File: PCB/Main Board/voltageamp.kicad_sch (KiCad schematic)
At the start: 45 parts, among them U601 INA828D, U602 DG201, U603 OPA2197xD, U604 DG201, U605 OPA2376xxD

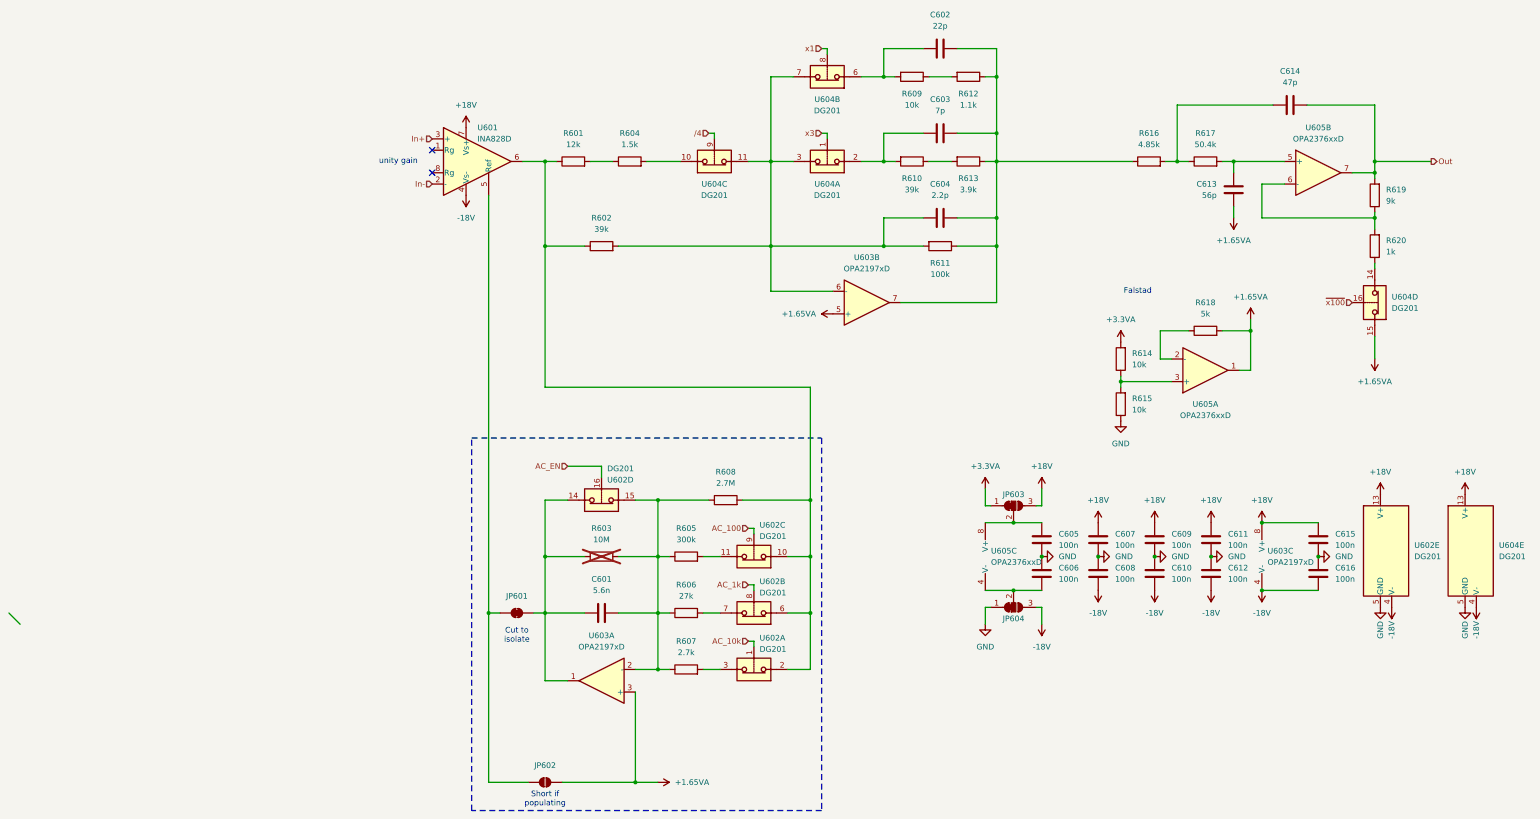
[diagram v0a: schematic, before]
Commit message: please be nice
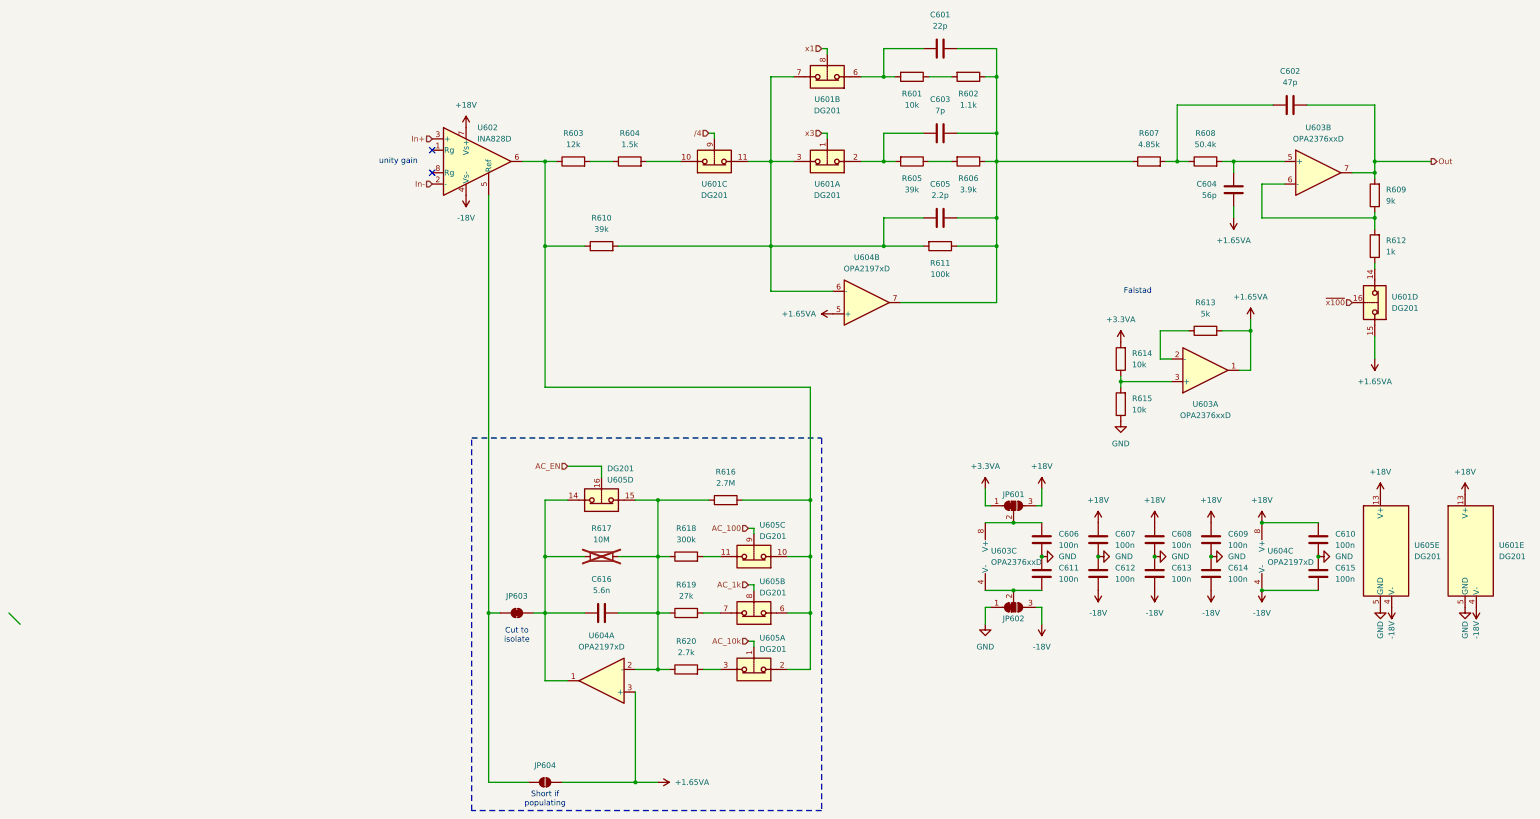
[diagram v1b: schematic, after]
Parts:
- renumbered C602 to C601, C614 to C602, C613 to C604, C604 to C605, C605 to C606, C609 to C608, C611 to C609, C615 to C610, C606 to C611, C608 to C612, C610 to C613, C612 to C614, C616 to C615, C601 to C616, JP603 to JP601, JP604 to JP602, JP601 to JP603, JP602 to JP604, R609 to R601, R612 to R602, R601 to R603, R610 to R605, R613 to R606, R616 to R607, R617 to R608, R619 to R609, R602 to R610, R620 to R612, R618 to R613, R608 to R616, R603 to R617, R605 to R618, R606 to R619, R607 to R620, U604 to U601, U601 to U602, U605 to U603, U603 to U604, U602 to U605

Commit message: hello
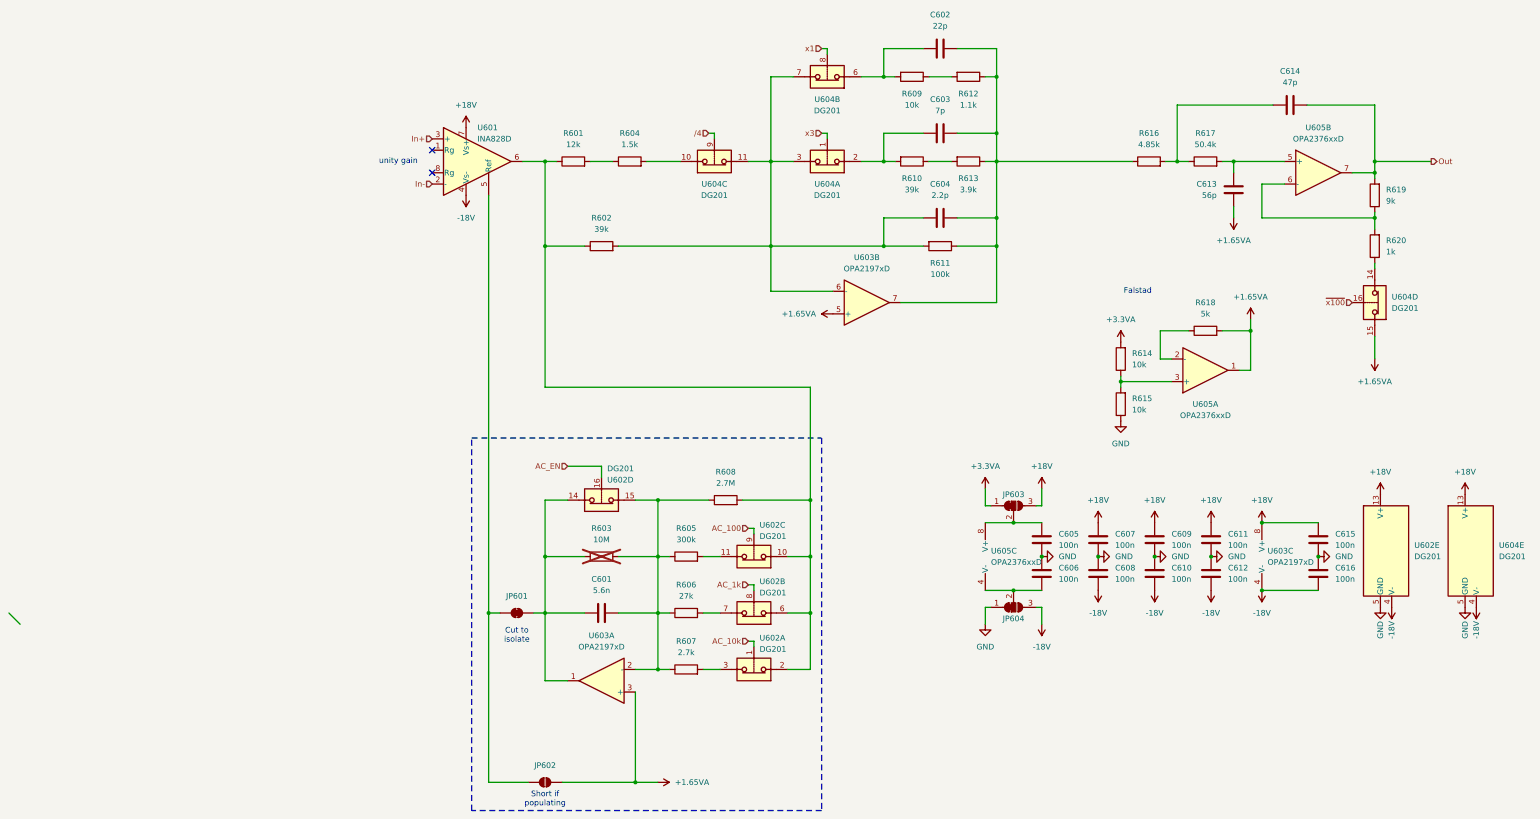
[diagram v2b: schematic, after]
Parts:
- renumbered C616 to C601, C601 to C602, C605 to C604, C606 to C605, C611 to C606, C612 to C608, C608 to C609, C613 to C610, C609 to C611, C614 to C612, C604 to C613, C602 to C614, C610 to C615, C615 to C616, JP603 to JP601, JP604 to JP602, JP601 to JP603, JP602 to JP604, R603 to R601, R610 to R602, R617 to R603, R618 to R605, R619 to R606, R620 to R607, R616 to R608, R601 to R609, R605 to R610, R602 to R612, R606 to R613, R607 to R616, R608 to R617, R613 to R618, R609 to R619, R612 to R620, U602 to U601, U605 to U602, U604 to U603, U601 to U604, U603 to U605
